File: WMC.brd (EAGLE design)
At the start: 110 x 115 mm, 64 parts, among them IC5 MCP2551, IC6 MCP2515, IC7 ATMEGA32U4NT-TQFP, J1 LEFT MOTOR, J10 XT30F, J11 USB-B-PTH, J12 RoboClaw, J2 RIGHT MOTOR, J3 M01-2.5MM, J4 M01-2.5MM, J5 M01-2.5MM, J6 M01-2.5MM, J7 M01-2.5MM, J8 M01-2.5MM, J9 XT30F, Q1 NTD5867NLT4G, Q2 NTD5867NLT4G

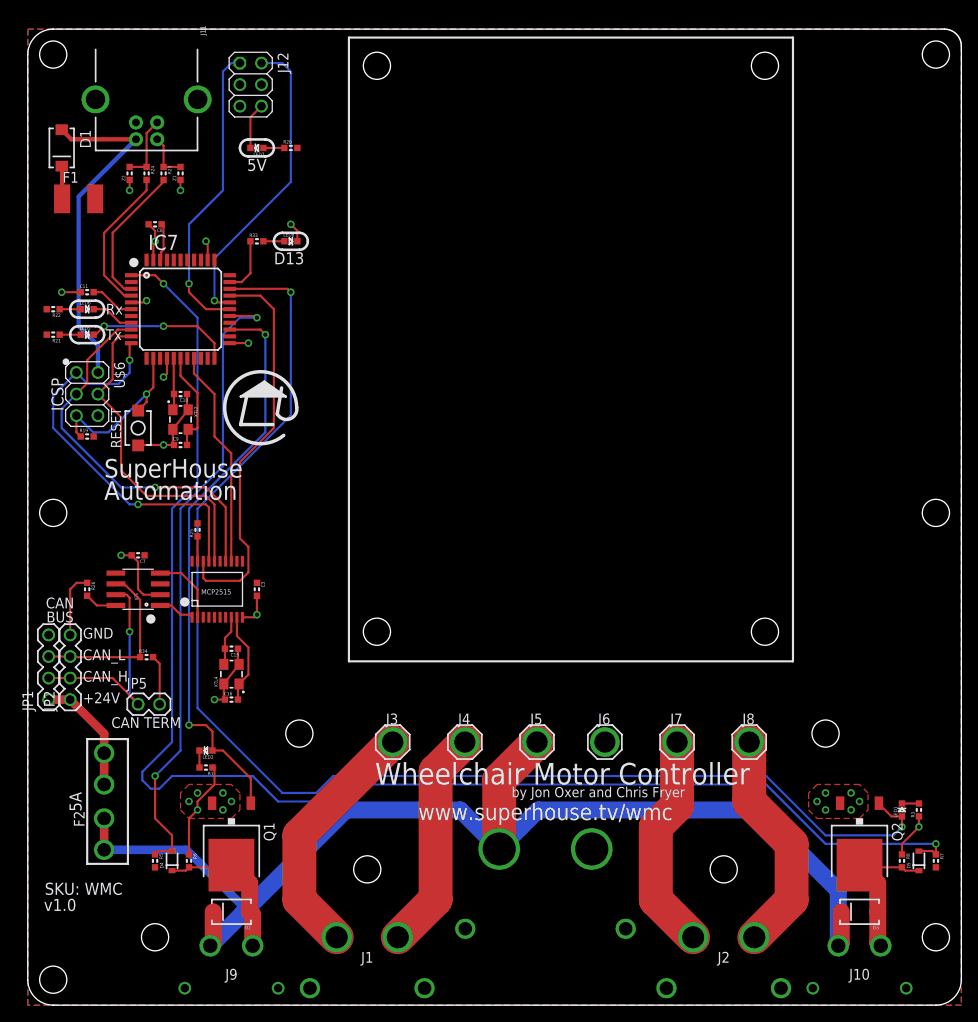
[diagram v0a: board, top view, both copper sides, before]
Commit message: Routing, ERC, DRC for v1.0 release
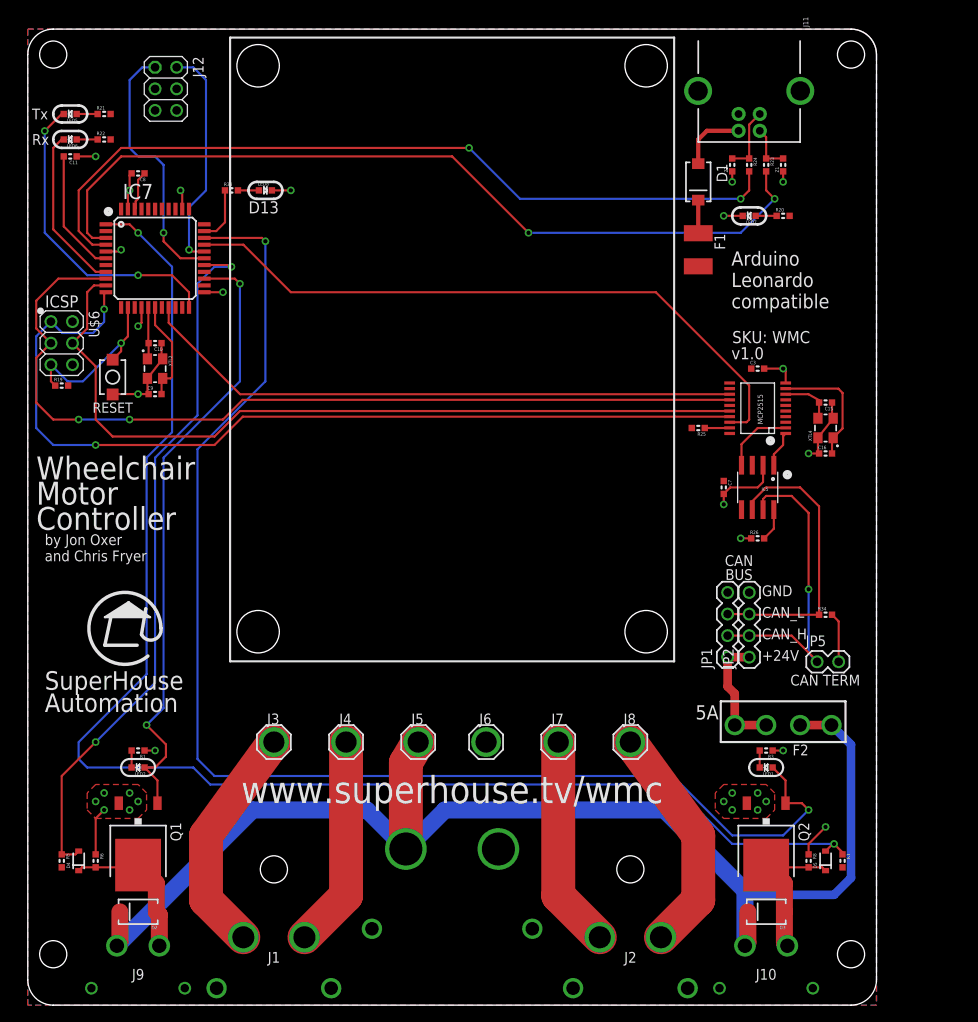
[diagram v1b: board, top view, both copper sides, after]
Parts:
- D2, D3: value (none) -> SS56
- D4, D5: value (none) -> 1N4148
- LED1, LED2: value (none) -> RED
- moved F2 80.5 mm to (89.0, 33.0), turned to 180 degrees
- moved JP1 80.2 mm to (82.5, 41.0)
- moved JP2 80.2 mm to (85.0, 41.0)
- moved JP5 80.2 mm to (93.0, 40.5)
- moved R34 80.2 mm to (94.0, 46.0)
- moved R26 79.2 mm to (86.0, 55.0), turned to 0 degrees
- moved C15 75.8 mm to (94.0, 71.0)
- moved C16 75.8 mm to (94.0, 65.0)
- moved XTL4 75.8 mm to (94.0, 68.0)
- moved D1 75.1 mm to (79.0, 97.0)
- moved IC5 74.0 mm to (86.0, 61.0), turned to 180 degrees
- moved F1 73.2 mm to (79.0, 89.0), turned to 270 degrees
- moved J11 71.0 mm to (85.0, 109.0)
- moved R23 71.0 mm to (87.0, 99.0)
- moved R24 71.0 mm to (85.0, 99.0)
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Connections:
- net 5V: now also U$6.2
- net USB+: no longer U$6.2
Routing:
- net RD-: track 16.7 -> 99.1 mm, vias 0 -> 2
- net RD+: track 17.5 -> 94.9 mm, vias 0 -> 2
- net MISO: track 47.2 -> 108.1 mm
- net SCK: track 45.5 -> 106.2 mm, vias 1 -> 2
- net MOSI: track 38.7 -> 96.1 mm
- net D2_SDA: track 25.7 -> 71.4 mm
- net USB+: track 40.4 -> 8.02 mm
- net D10_A11: track 46.8 -> 77.5 mm
- net TX_LED: track 17.3 -> 36.8 mm
- net GND: track 82.0 -> 67.2 mm, vias 26 -> 30
- net RXLED_SS: track 5.10 -> 19.5 mm
- net CANL: track 21.2 -> 34.0 mm
- net 24V: track 141.3 -> 152.3 mm
- net CANH: track 26.6 -> 37.4 mm
- net D9_A10: track 36.5 -> 26.8 mm
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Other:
- board size 110 x 115 mm -> 100 x 115 mm
- board text added: "Arduino Leonardo compatible"
- board text removed: "5V"
